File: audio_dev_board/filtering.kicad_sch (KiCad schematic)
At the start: 11 parts, among them U4 TL072, U5 TL072

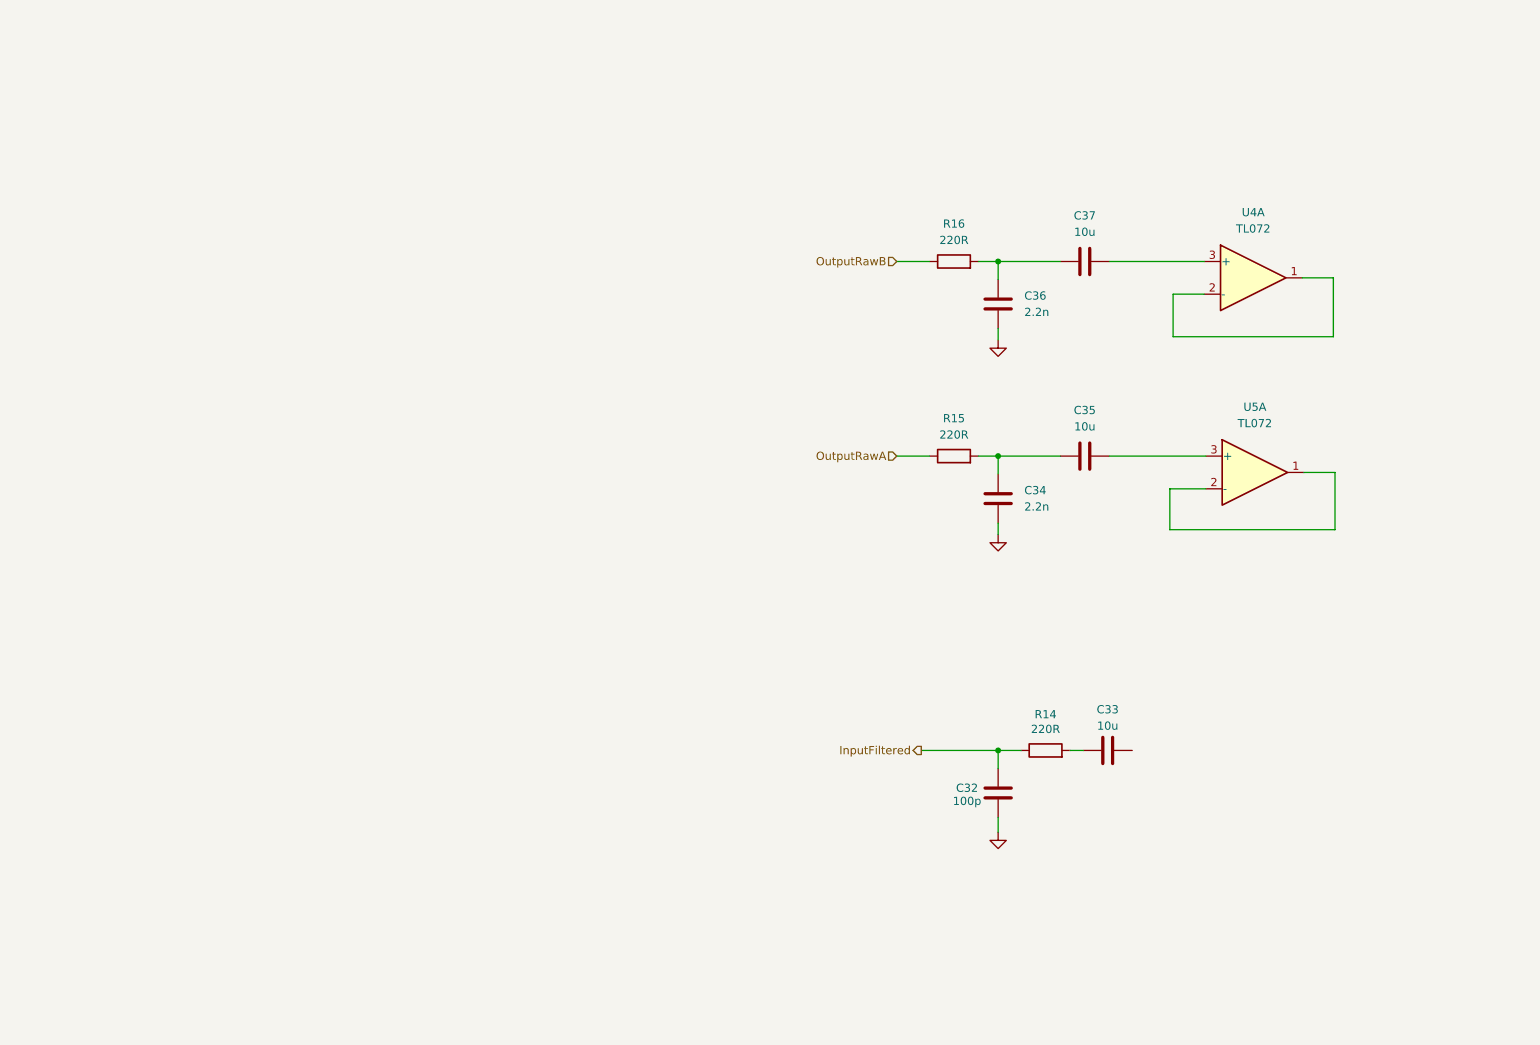
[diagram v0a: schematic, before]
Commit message: bluhhh
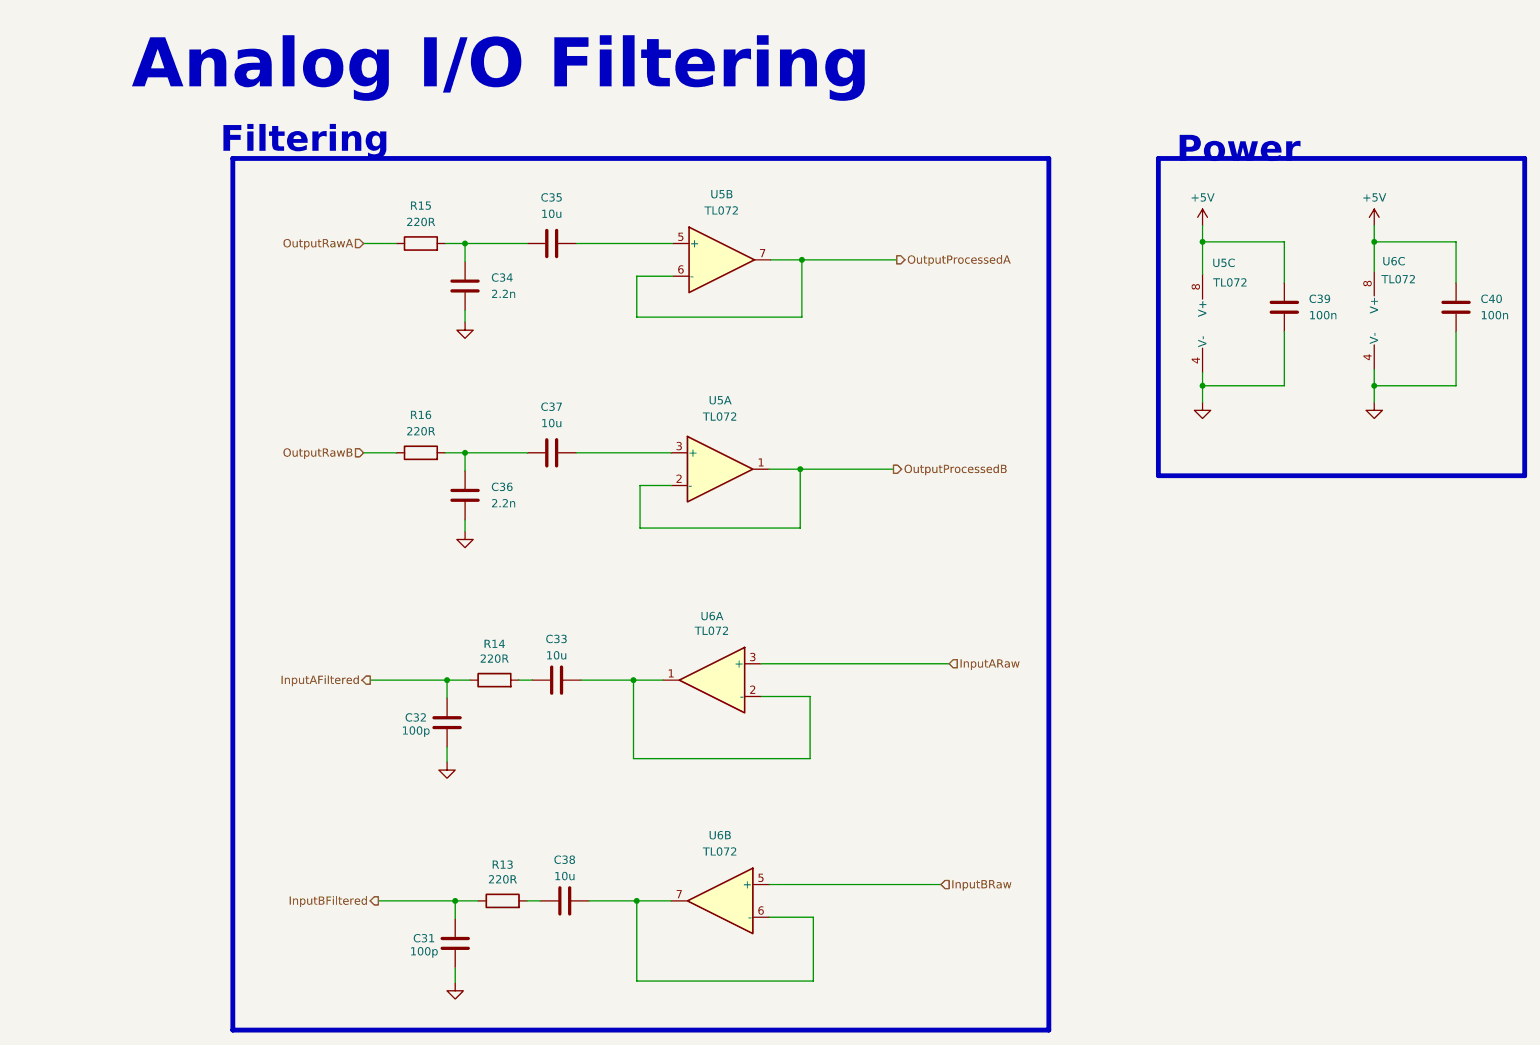
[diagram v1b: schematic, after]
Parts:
- added C31: 100p, symbol Device:C
- added C38: 10u, symbol Device:C
- added C39, C40: 100n, symbol Device:C
- added R13: 220R, symbol Device:R
- added unit 3 of U5
- added U6: TL072, symbol Amplifier_Operational:TL072
- renumbered U4 to U5
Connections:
- net GND: now also C31.1, C39.2, C40.2, U5.4 (V-), U6.4 (V-)
- net at C35.2: now also U5.5 (+); no longer U5.3 (+)
- net at C33.2: now also U6.1, U6.2 (-)
- net OutputProcessedB: now reaches U5.1, U5.2 (-)
- net InputFiltered renamed InputAFiltered
- new net: C38.2, U6.6 (-), U6.7
- new net: C38.1, R13.2
- new net +5V: C39.1, C40.1, U5.8 (V+), U6.8 (V+)
- new net InputARaw: U6.3 (+)
- new net InputBFiltered: C31.2, R13.1
- new net InputBRaw: U6.5 (+)
- new net OutputProcessedA: U5.6 (-), U5.7
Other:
- note added: "Analog I/O Filtering"
- note added: "Filtering"
- note added: "Power"
- moved on the sheet: C32, C33, C34, C35, C36, C37, R14, R15, R16, U5A, U5B
